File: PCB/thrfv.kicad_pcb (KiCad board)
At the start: 2 copper layers, 126.3 x 98.6 mm, 84 parts, among them J1 4PIN, J2 OLED, J3 Conn_01x05_Female, J4 Conn_01x05_Female, SW1 SW1, SW10 SW10, SW11 SW11, SW12 SW12, SW13 SW13, SW14 SW14, SW15 SW15, SW16 SW_Contact_Pad, SW17 SW_Contact_Pad, SW18 SW18, SW19 SW19, SW2 SW2, SW20 SW20, SW3 SW3, SW4 SW4, SW5 SW5, SW6 SW6, SW7 SW7, SW8 SW8, SW9 SW9, U1 ProMicro

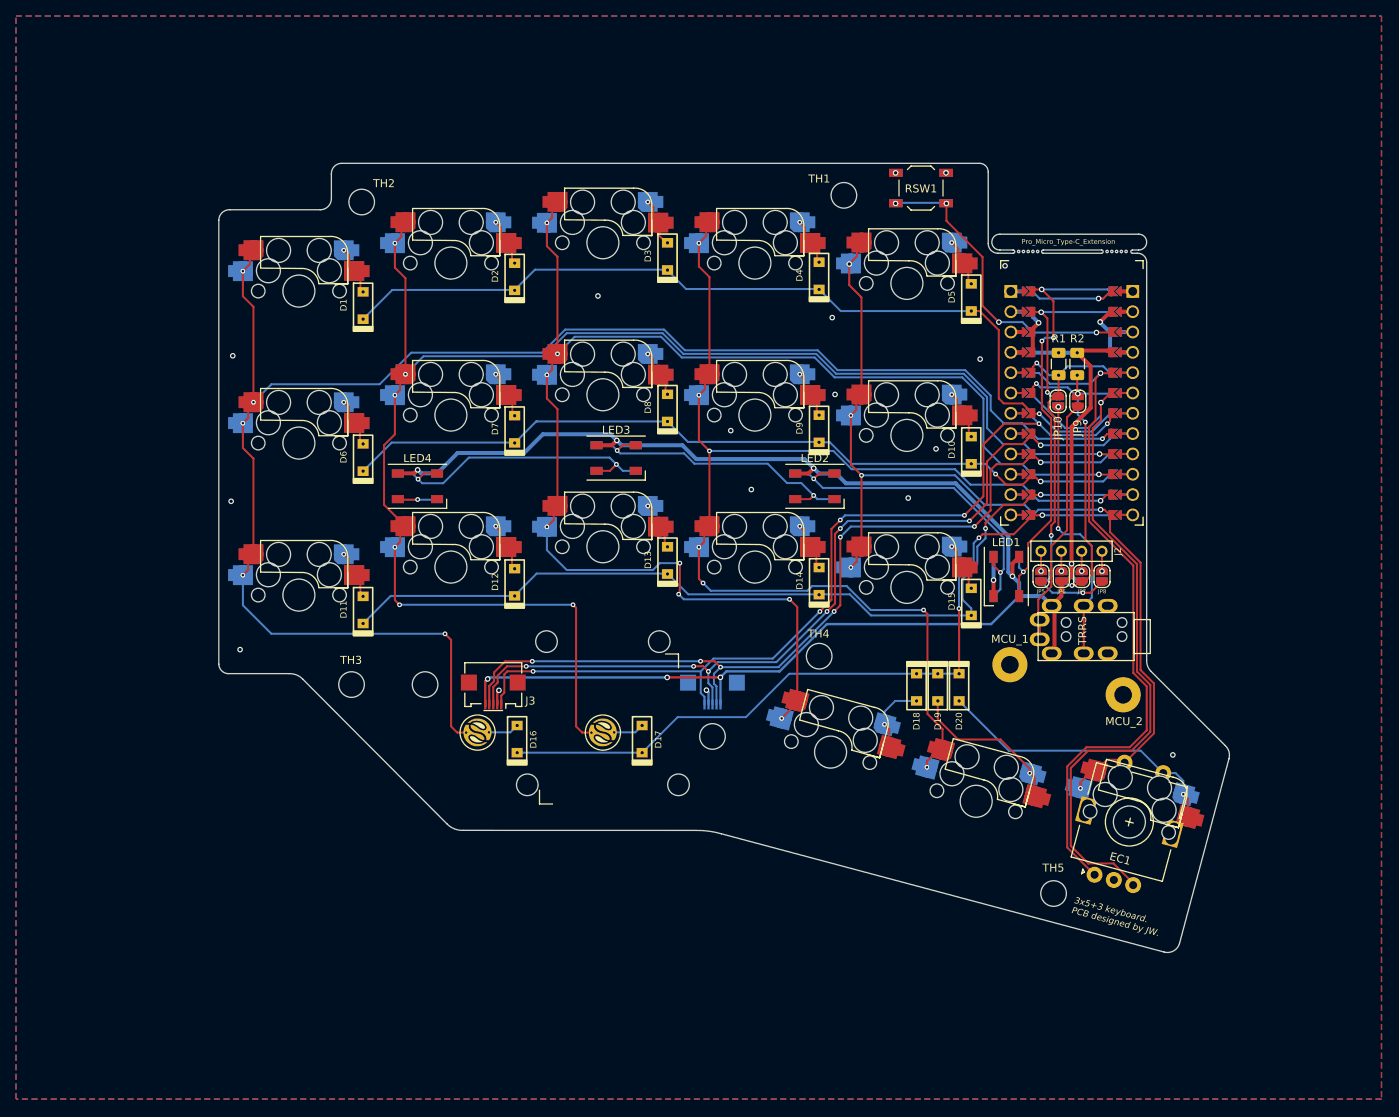
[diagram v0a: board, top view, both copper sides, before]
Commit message: No comment.
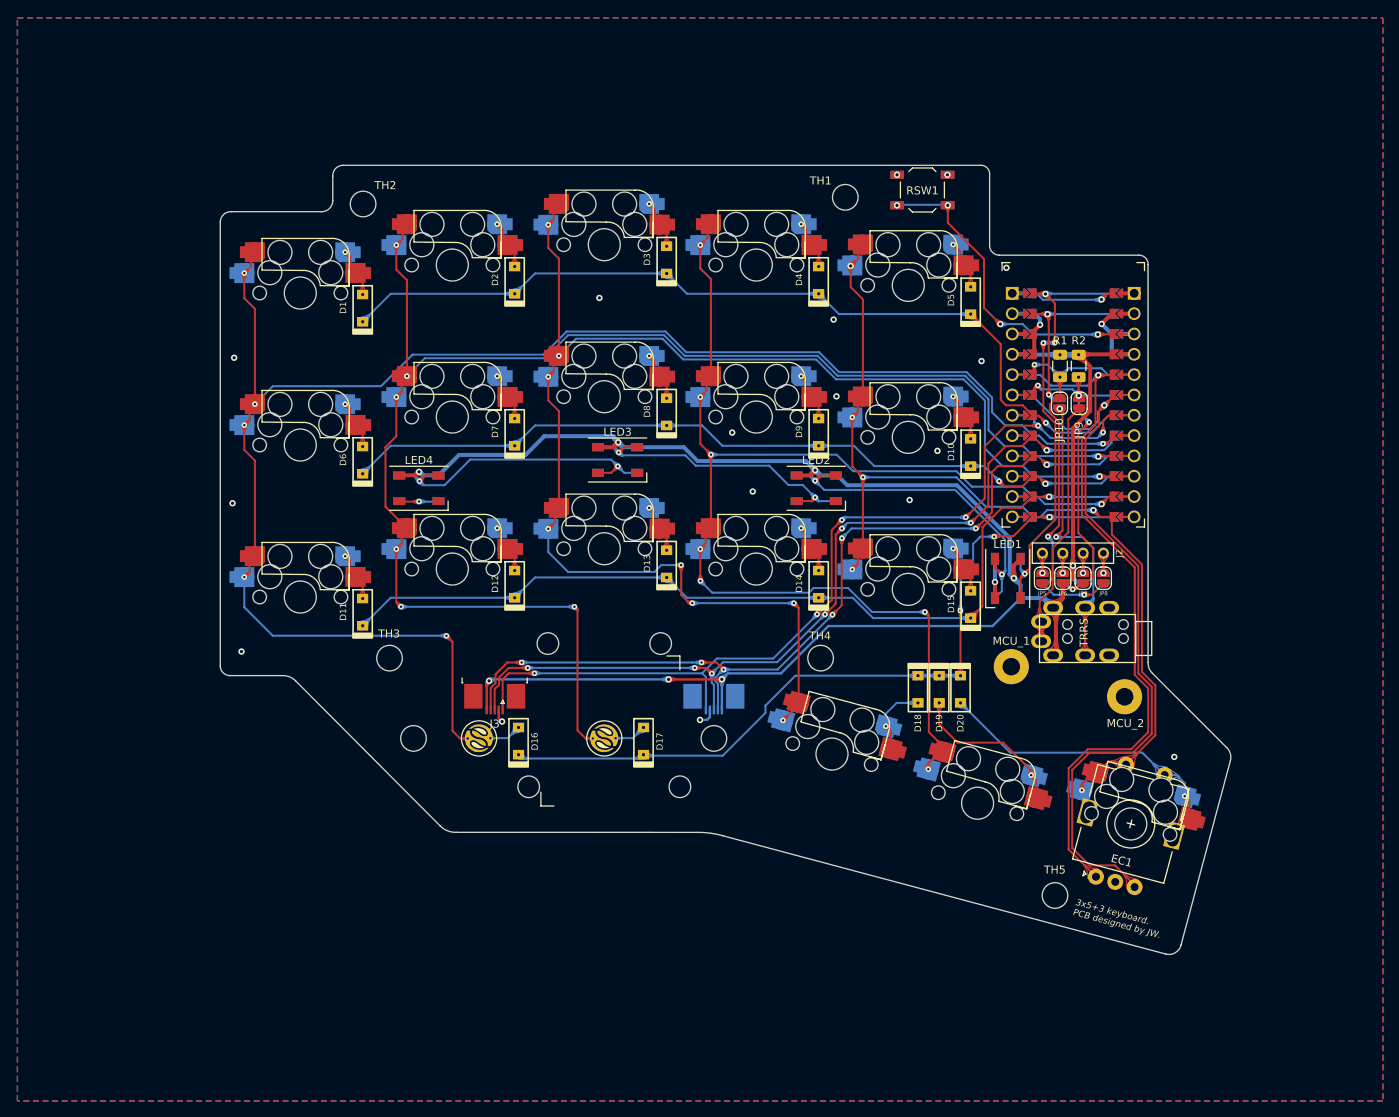
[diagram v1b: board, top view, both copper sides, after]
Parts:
- removed the REF** at (199.1, 69.6)
- removed the REF** at (210.1, 69.6)
- removed the REF** at (145.9, 129.2) (x2)
- added REF**: Nintendo_Switch_JOYSTICK, jw_custom_footprint:Nintendo_Switch_JOYSTICK, F.Cu at (146.1, 129.5)
- added REF**: Nintendo_Switch_JOYSTICK, jw_custom_footprint:Nintendo_Switch_JOYSTICK, B.Cu at (146.1, 129.5)
- J3, J4: footprint jw_custom_footprint:Molex_200528-0050_1x05-1MP_P0.5mm_Horizontal -> Connector_FFC-FPC:TE_0-1734839-5_1x05-1MP_P0.5mm_Horizontal
- moved JY_BT_1 6.88 mm to (122.3, 130.4)
- moved TH3 5.78 mm to (119.3, 120.4)
- moved SW17 0.75 mm to (146.1, 130.4)
- moved SW16 0.75 mm to (130.5, 130.4)
- moved D4 0.55 mm to (172.9, 73.1)
- moved D8 0.51 mm to (153.9, 89.6)
- moved D13 0.44 mm to (153.9, 108.6)
- moved D3 0.44 mm to (153.9, 70.6)
- moved D9 0.43 mm to (172.9, 92.1)
- moved D2 0.43 mm to (134.9, 73.1)
- moved D5 0.39 mm to (191.9, 75.7)
- moved D14 0.38 mm to (172.9, 111.1)
- moved D7 0.35 mm to (134.9, 92.1)
- moved D15 0.34 mm to (191.9, 113.7)
- moved D1 0.33 mm to (115.9, 76.6)
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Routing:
- net Net-(D8-Pad2): track 3.42 -> 5.21 mm
- net Net-(D4-Pad2): track 3.42 -> 5.21 mm
- net Net-(D13-Pad2): track 3.34 -> 5.06 mm
- net Net-(D9-Pad2): track 3.39 -> 5.06 mm
- net Net-(D5-Pad2): track 3.85 -> 5.49 mm
- net Net-(D14-Pad2): track 3.44 -> 5.06 mm
- net Net-(D2-Pad2): track 3.66 -> 5.28 mm
- net Net-(D15-Pad2): track 3.61 -> 5.21 mm
- net Net-(D1-Pad2): track 3.71 -> 5.28 mm
- net Net-(D6-Pad2): track 3.64 -> 5.21 mm
- net Net-(D10-Pad2): track 3.66 -> 5.21 mm
- net Net-(D7-Pad2): track 3.52 -> 5.06 mm
- net Net-(D11-Pad2): track 3.62 -> 5.14 mm
- net Net-(D12-Pad2): track 3.65 -> 5.06 mm
- net Net-(J1-Pad2): track 34.2 -> 35.6 mm
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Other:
- outline, holes or cut-outs redrawn
- board text removed: "Pro_Micro_Type-C_Extension"
